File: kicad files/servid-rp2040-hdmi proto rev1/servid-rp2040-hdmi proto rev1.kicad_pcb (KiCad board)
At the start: 2 copper layers, 81 parts, among them J1 ITU-656, J10 SYNCs, J11 SPKR, J2 INT_LA, J3 I2C_LA, J4 SND_LA, J5 USB_B_Micro-CHECK FOOTPRINT, J6 VIDS, J7 10029449-111RLF-CHANGE FOOTPR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, J8 SWD, J9 GPIO, SW1 RP_RST, U1 RP2040, U2 MIC5504-3.3YM5, U3 MIC5504-3.3YM5, U4 MIC5504-1.8YM5, U5 IT6613, U6 MIC5504-1.8YM5, U7 W25Q128JVS, Y1 ECS-120-18-33-JEM

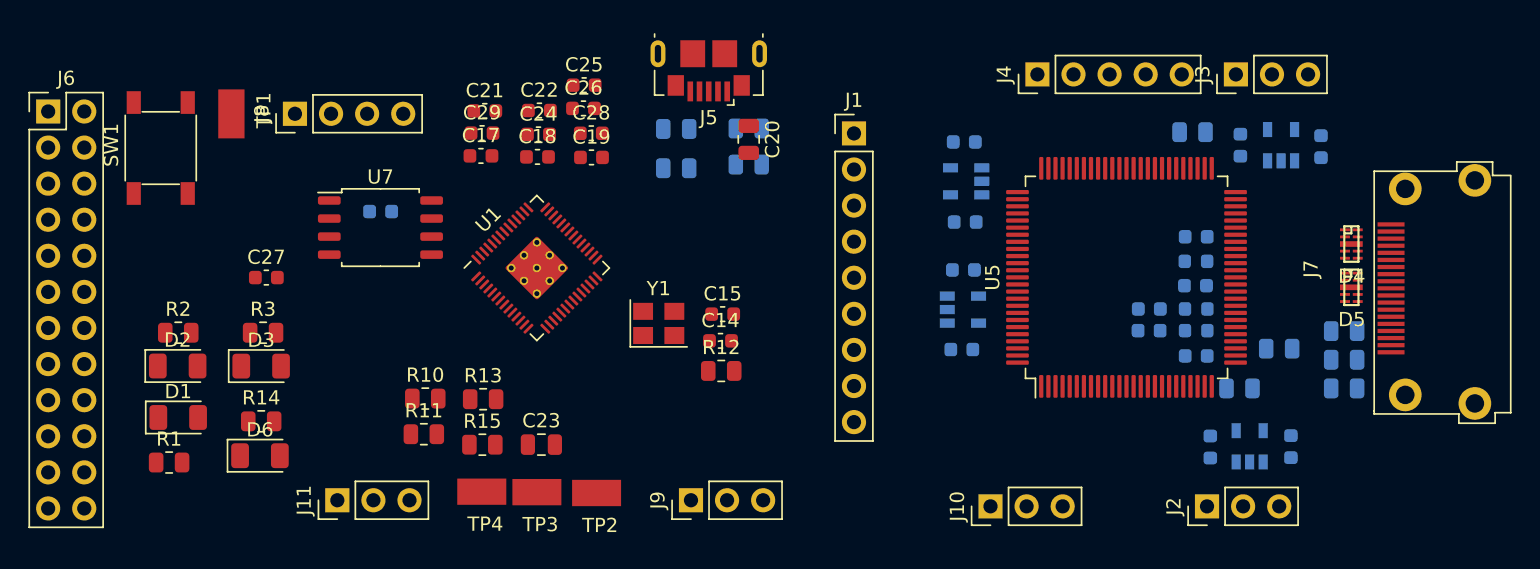
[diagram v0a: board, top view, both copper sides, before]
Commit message: critical routes
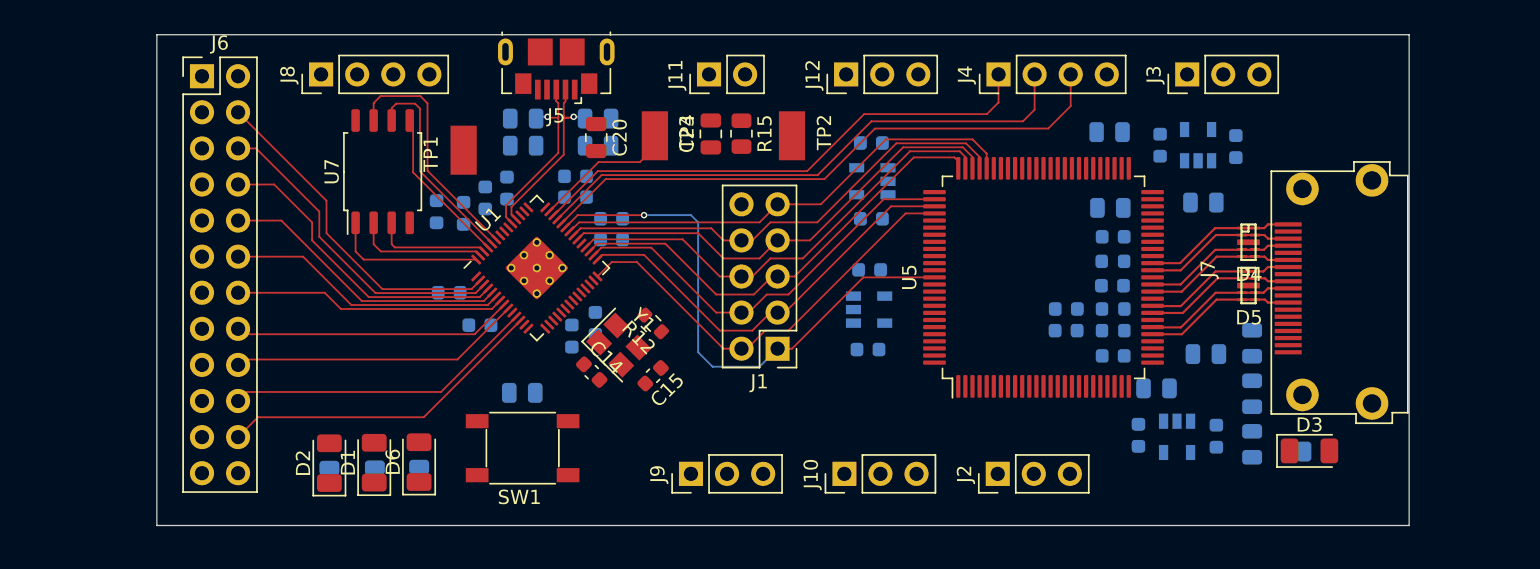
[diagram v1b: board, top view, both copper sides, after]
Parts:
- removed TP3: TP_SPKR_ADC, My Libraries:Harwin-S1751-46-Test-Point
- added J12: PWR, Connector_PinHeader_2.54mm:PinHeader_1x03_P2.54mm_Vertical, F.Cu at (170.4, 122.4)
- C17, C18, C19, C21, C22, C24, C25, C26, C27, C28, C29, R1, R10, R11, R13, R14, R2, R3: moved to B.Cu
- J1: footprint Connector_PinHeader_2.54mm:PinHeader_1x09_P2.54mm_Vertical -> Connector_PinHeader_2.54mm:PinHeader_2x05_P2.54mm_Vertical
- J11: footprint Connector_PinHeader_2.54mm:PinHeader_1x03_P2.54mm_Vertical -> Connector_PinHeader_2.54mm:PinHeader_1x02_P2.54mm_Vertical
- J4: footprint Connector_PinHeader_2.54mm:PinHeader_1x05_P2.54mm_Vertical -> Connector_PinHeader_2.54mm:PinHeader_1x04_P2.54mm_Vertical
- R12: footprint Resistor_SMD:R_0805_2012Metric -> Resistor_SMD:R_0603_1608Metric
- moved R3 74.7 mm to (203.6, 149.0)
- moved D3 74.0 mm to (203.0, 148.9)
- moved R10 56.5 mm to (195.6, 131.4), turned to 180 degrees
- moved R11 50.9 mm to (189.0, 131.8)
- moved J11 39.8 mm to (160.8, 122.4)
- moved SW1 33.1 mm to (147.7, 148.7), turned to 180 degrees
- moved TP2 28.7 mm to (166.6, 126.7), turned to 90 degrees
- moved R15 28.5 mm to (163.1, 126.6), turned to 270 degrees
- moved TP4 27.9 mm to (157.0, 126.7), turned to 90 degrees
- moved C23 24.9 mm to (160.9, 126.6), turned to 90 degrees
- moved C25 17.7 mm to (151.1, 140.8), turned to 270 degrees
- moved TP1 16.5 mm to (143.5, 127.8), turned to 270 degrees
- moved C27 16.4 mm to (145.0, 131.1), turned to 90 degrees
- moved J1 16.1 mm to (165.6, 141.7), turned to 180 degrees
- moved C22 15.7 mm to (144.7, 140.1), turned to 180 degrees
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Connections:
- net Net-(R13-Pad1) renamed /Run
- J1 pad 1: /CY0 -> /PxCLK
- J1 pad 2: /CY1 -> /CY0
- J1 pad 3: /CY2 -> /CY1
- J1 pad 4: /CY3 -> /CY2
- J1 pad 5: /CY4 -> /CY3
- J1 pad 6: /CY5 -> /CY4
- J1 pad 7: /CY6 -> /CY5
- J1 pad 8: /CY7 -> /CY6
- J1 pad 9: /PxCLK -> /CY7
- J11 pad 2: /SPKR_ADC -> /SPKR_IN
- J4 pad 1: /PIO_I2S_CLK -> /PIO_I2S_WS
- J4 pad 3: /PIO_I2S_WS -> /PIO_I2S_CLK
- J4 pad 4: /SPKR_IN -> GND
- U1 pad 41: /SPKR_ADC -> /SPKR_RC
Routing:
- net /PIO_I2S_CLK: track 0.00 -> 41.5 mm
- net /PIO_I2S_DATA: track 0.00 -> 39.3 mm
- net /PxCLK: track 0.00 -> 38.7 mm, vias 0 -> 1
- net /PIO_I2S_WS: track 0.00 -> 36.6 mm
- net /CY7: track 0.00 -> 33.5 mm
- net /CY6: track 0.00 -> 33.2 mm
- net /CY5: track 0.00 -> 33.0 mm
- net /CY4: track 0.00 -> 32.7 mm
- net /CY3: track 0.00 -> 32.3 mm
- net /CY0: track 0.00 -> 30.6 mm
- net /CY1: track 0.00 -> 29.7 mm
- net /CY2: track 0.00 -> 29.4 mm
- net /14M: track 0.00 -> 23.8 mm
- net /~SYNC: track 0.00 -> 23.3 mm
- net /7M: track 0.00 -> 22.8 mm
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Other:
- board outline added: 88.1 x 34.5 mm
- copper layers 2 -> 4
- net class Default: clearance 0.2 -> 0.1524; trace_width 0.25 -> 0.127; via_dia 0.8 -> 0.4572; via_drill 0.4 -> 0.254
- rule pad_to_mask_clearance: 0 -> 0.0508
- rule trace_clearance: 0.2 -> 0.1524
- rule trace_min: 0.2 -> 0.127
- rule via_min_drill: 0.3 -> 0.254
- rule via_min_size: 0.4 -> 0.4572
